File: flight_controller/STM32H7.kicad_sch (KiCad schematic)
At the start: 65 parts, among them SW1 6.0*6.0*6.0, U1 HB-PH9-12727PB2GOB, U2 STM32H743IIT6, X1 XKXEL89CLI-SUAYLC-32.768K, X2 XL2EL89CLI-111YLC-16M

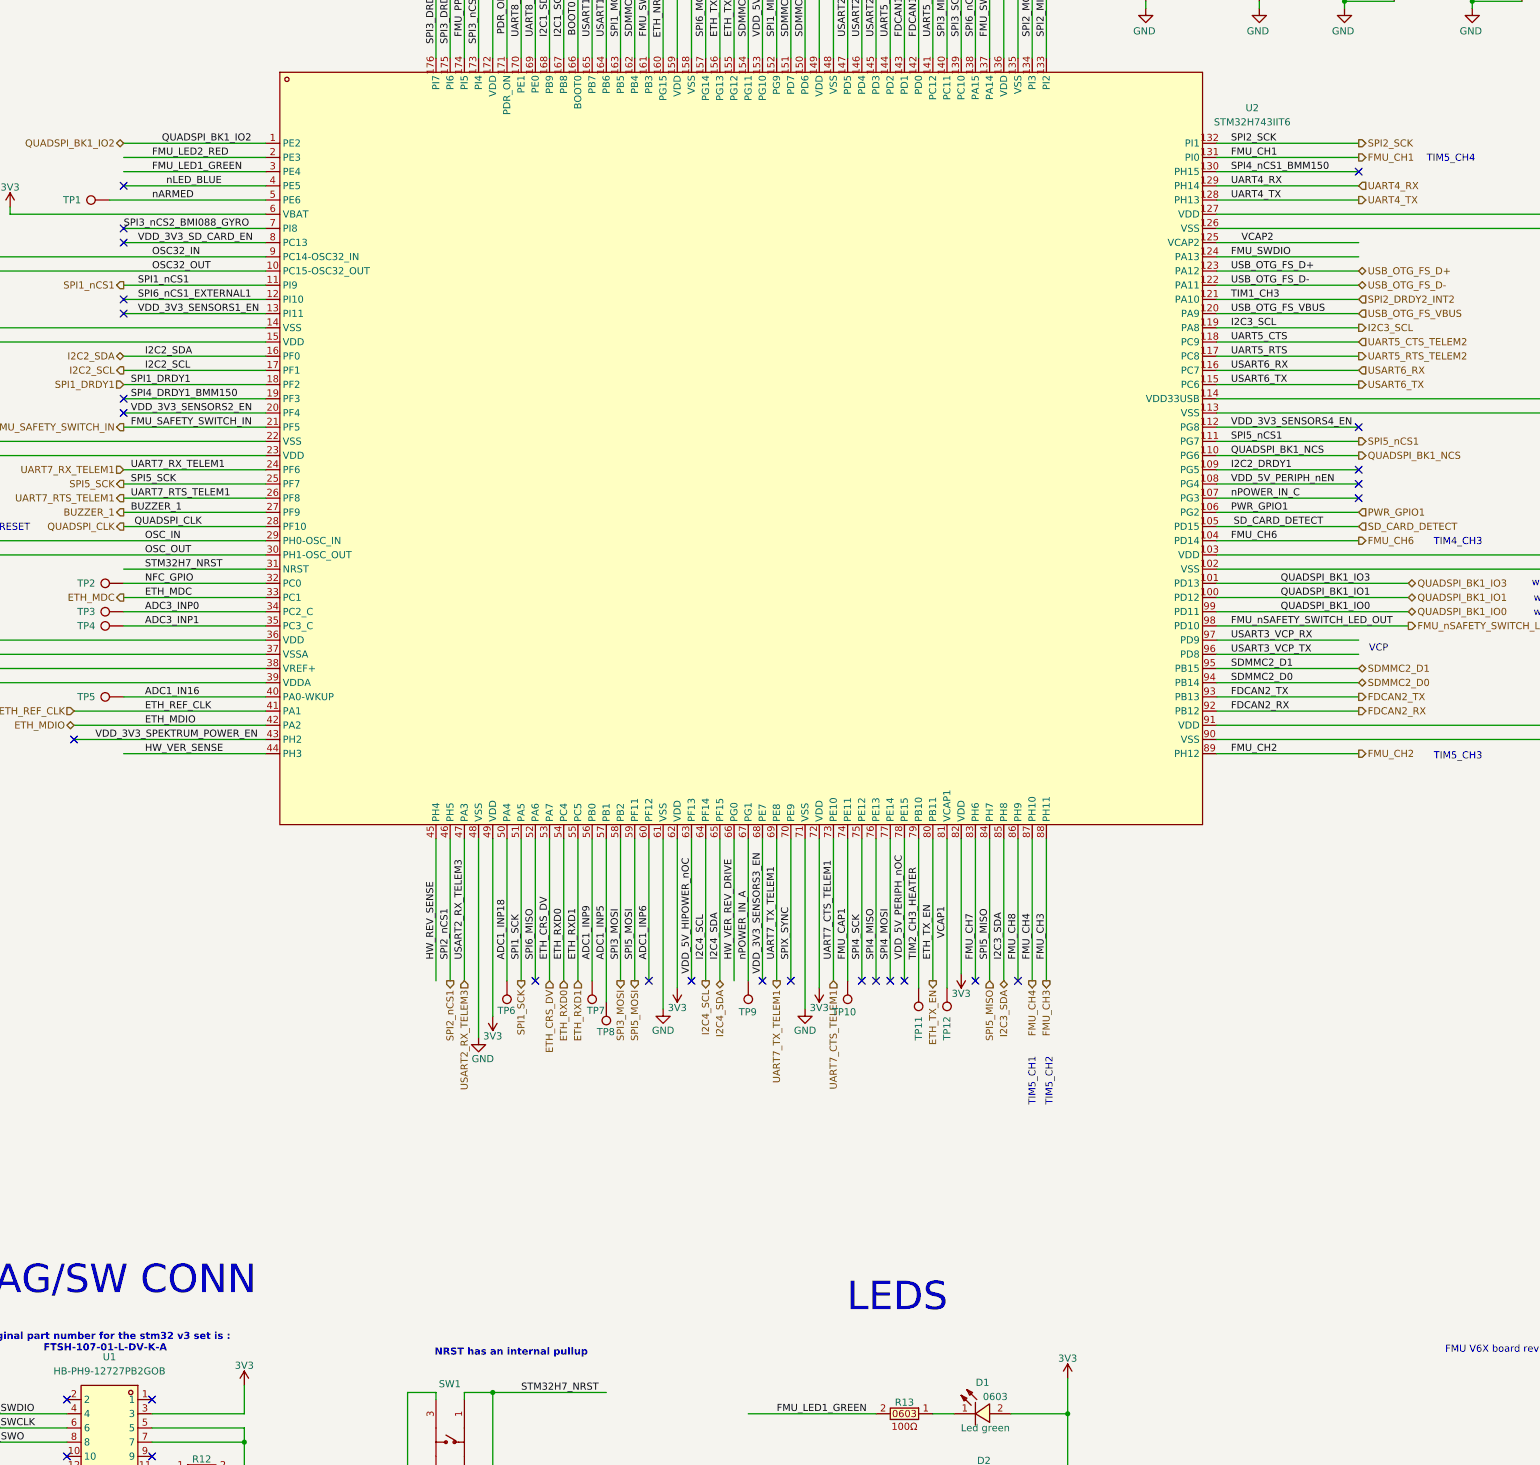
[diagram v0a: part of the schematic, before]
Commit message: Updated power and usb connectors, annotations and netlist check
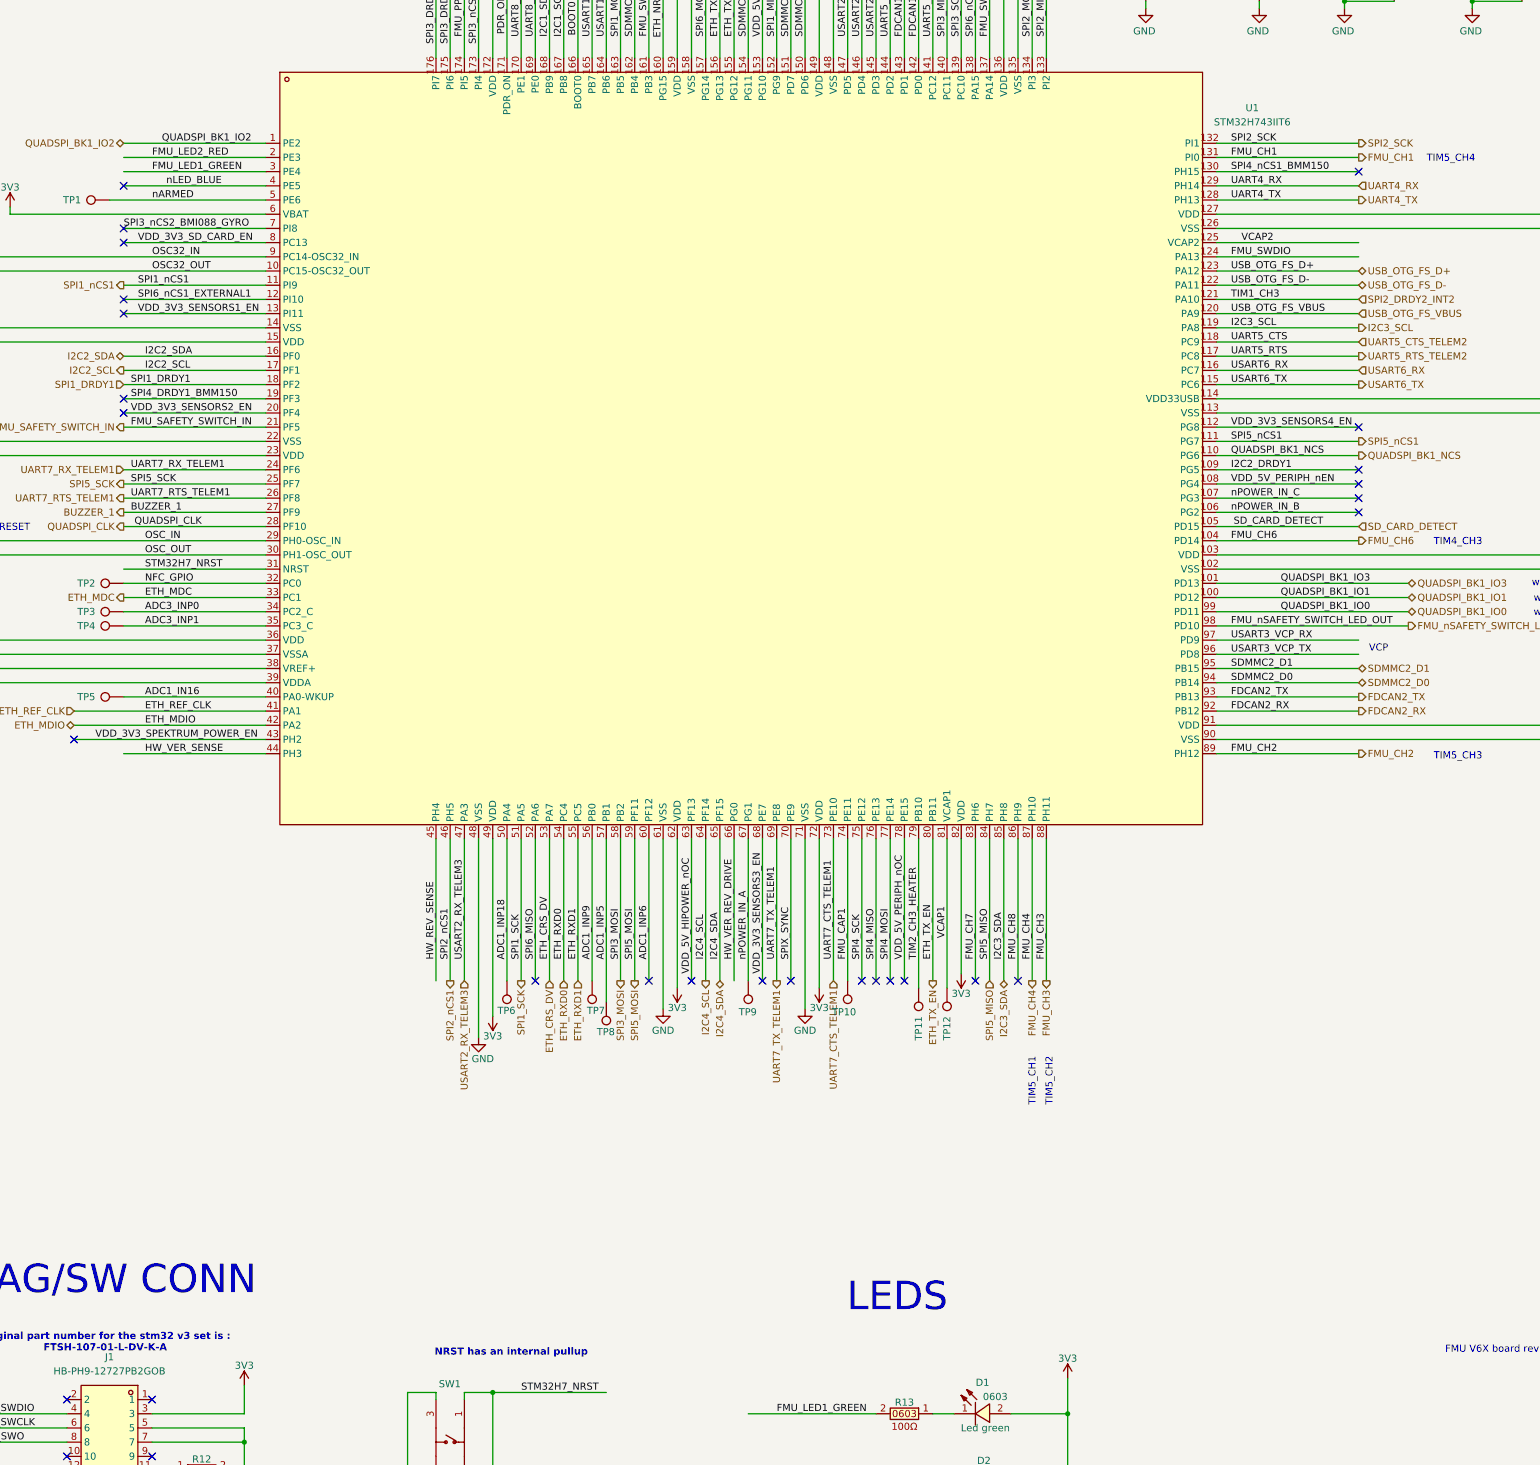
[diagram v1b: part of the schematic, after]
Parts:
- renumbered U1 to J1, U2 to U1
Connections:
- net PWR_GPIO1 renamed nPOWER_IN_B
- no-connect marks 35 -> 36
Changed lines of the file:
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@@
 	)
 	(no_connect
+		(at 511.81 186.69)
+	)
+	(no_connect
 		(at 290.83 166.37)
 	)
@@
 			(width 0)
 			(type default)
+			(color 255 0 0 1)
 		)
 	)
@@
 		)
 	)
-	(label "PWR_GPIO1"
-		(at 488.95 186.69 0)
-		(effects
-			(font
-				(size 1.27 1.27)
-			)
-			(justify left bottom)
-		)
-	)
 	(label "UART5_RX"
 		(at 427.99 101.6 90)
@@
 		)
 	)
+	(label "nPOWER_IN_B"
+		(at 488.95 186.69 0)
+		(effects
+			(font
+				(size 1.27 1.27)
+			)
+			(justify left bottom)
+		)
+	)
 	(label "FMU_SWCLK"
 		(at 445.77 101.6 90)
@@
 		)
 	)
-	(hierarchical_label "PWR_GPIO1"
-		(shape input)
-		(at 511.81 186.69 0)
-		(effects
-			(font
-				(size 1.27 1.27)
-			)
-			(justify left)
-		)
-	)
 	(hierarchical_label "FMU_CH1"
 		(shape output)
@@
 		(on_board yes)
 		(dnp no)
-		(property "Reference" "U1"
+		(property "Reference" "J1"
 			(at 288.29 337.82 0)
 			(effects
@@
 			(project "FP_BOARD"
 				(path "/17737359-1a8e-4237-8899-d9604030bc1d/21c4e215-368e-4a6b-9b68-3566112ef4e7"
-					(reference "U1")
+					(reference "J1")
 					(unit 1)
 				)
@@
 		(dnp no)
 		(fields_autoplaced yes)
-		(property "Reference" "U2"
+		(property "Reference" "U1"
 			(at 492.76 114.3314 0)
 			(effects
@@
 			(project "FP_BOARD"
 				(path "/17737359-1a8e-4237-8899-d9604030bc1d/21c4e215-368e-4a6b-9b68-3566112ef4e7"
-					(reference "U2")
+					(reference "U1")
 					(unit 1)
 				)

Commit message: Revert to state of commit 2458262 moved all to components to top
Reverts commits: d012532, 3d9c600, 58bc0ac
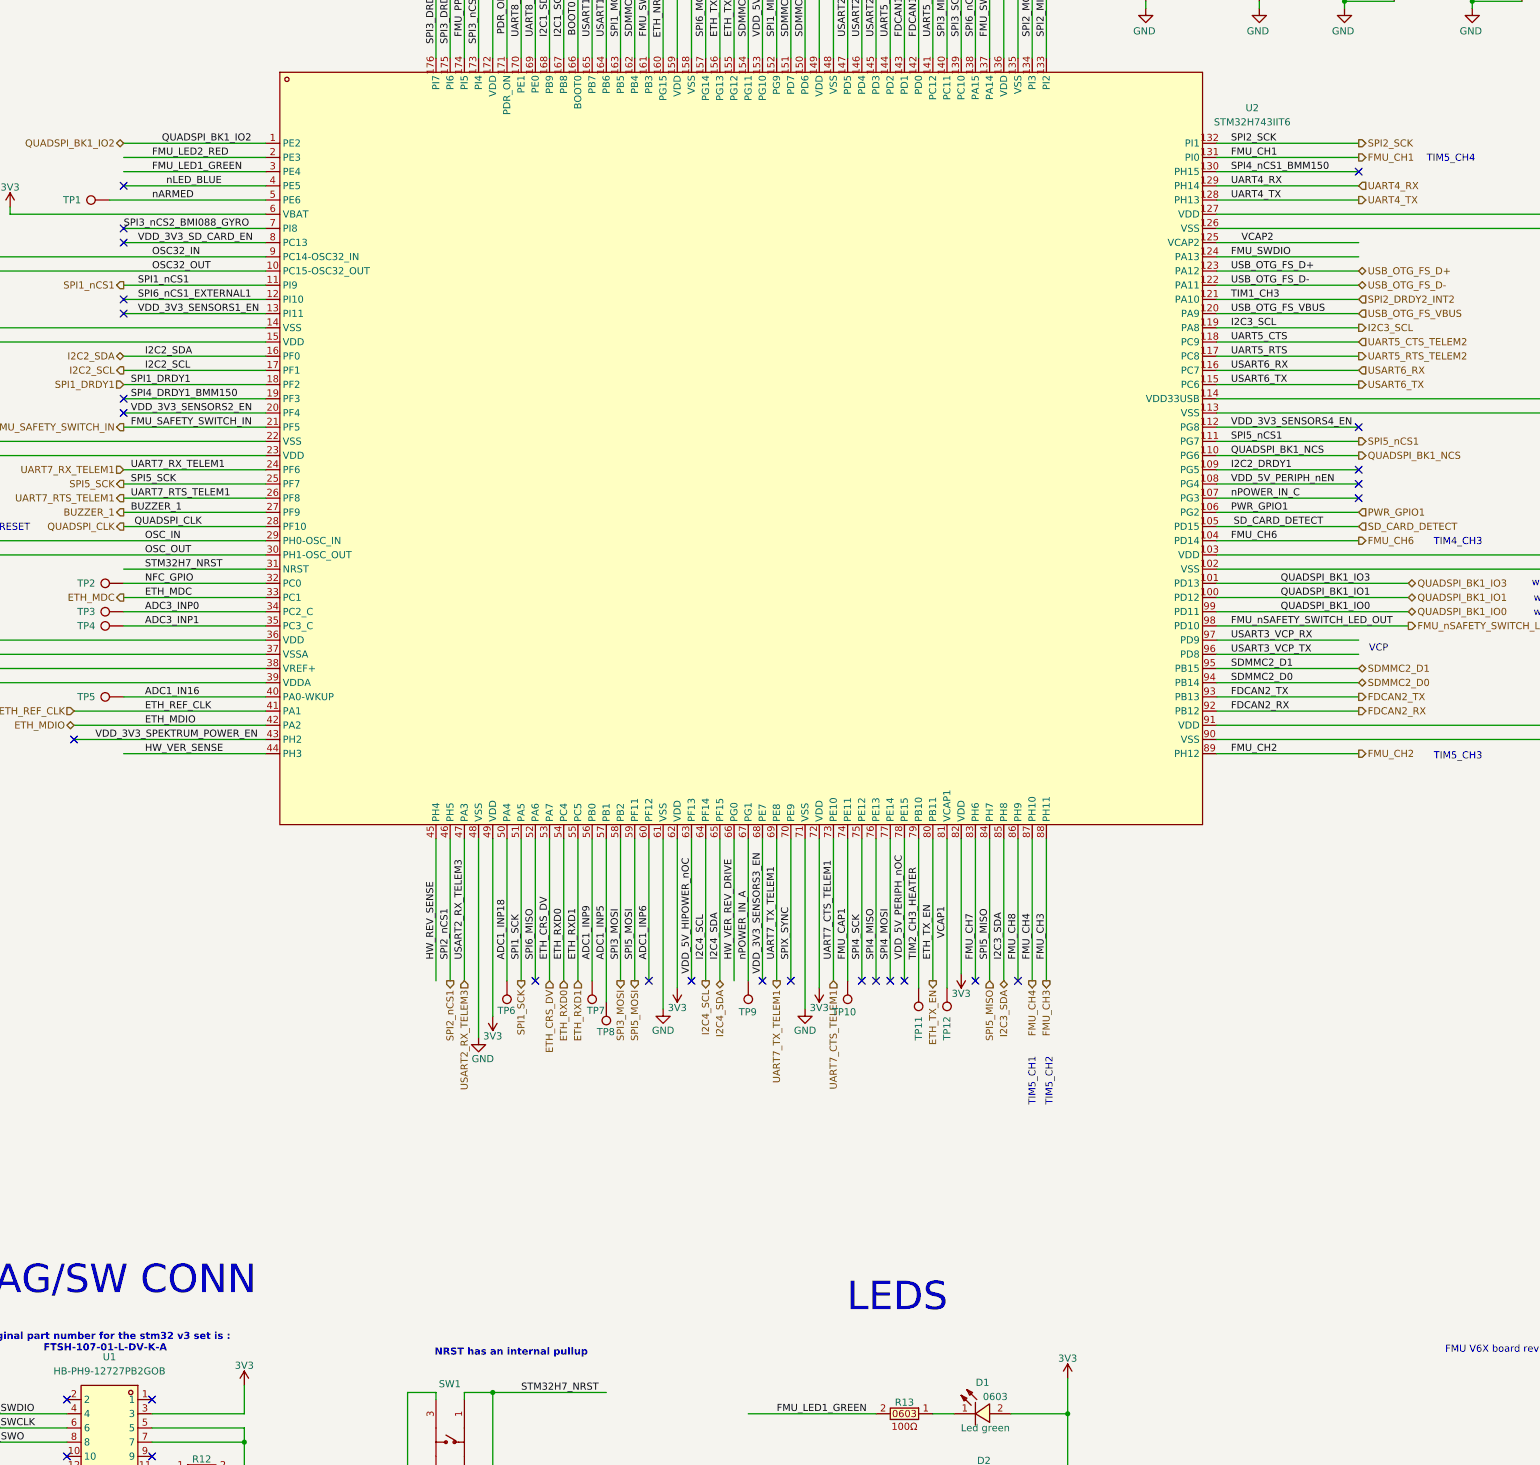
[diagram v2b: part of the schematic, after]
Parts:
- renumbered J1 to U1, U1 to U2
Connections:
- net nPOWER_IN_B renamed PWR_GPIO1
- no-connect marks 36 -> 35
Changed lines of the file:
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@@
 	)
 	(no_connect
-		(at 511.81 186.69)
-	)
-	(no_connect
 		(at 290.83 166.37)
 	)
@@
 			(width 0)
 			(type default)
-			(color 255 0 0 1)
 		)
 	)
@@
 		)
 	)
+	(label "PWR_GPIO1"
+		(at 488.95 186.69 0)
+		(effects
+			(font
+				(size 1.27 1.27)
+			)
+			(justify left bottom)
+		)
+	)
 	(label "UART5_RX"
 		(at 427.99 101.6 90)
@@
 		)
 	)
-	(label "nPOWER_IN_B"
-		(at 488.95 186.69 0)
-		(effects
-			(font
-				(size 1.27 1.27)
-			)
-			(justify left bottom)
-		)
-	)
 	(label "FMU_SWCLK"
 		(at 445.77 101.6 90)
@@
 		)
 	)
+	(hierarchical_label "PWR_GPIO1"
+		(shape input)
+		(at 511.81 186.69 0)
+		(effects
+			(font
+				(size 1.27 1.27)
+			)
+			(justify left)
+		)
+	)
 	(hierarchical_label "FMU_CH1"
 		(shape output)
@@
 		(on_board yes)
 		(dnp no)
-		(property "Reference" "J1"
+		(property "Reference" "U1"
 			(at 288.29 337.82 0)
 			(effects
@@
 			(project "FP_BOARD"
 				(path "/17737359-1a8e-4237-8899-d9604030bc1d/21c4e215-368e-4a6b-9b68-3566112ef4e7"
-					(reference "J1")
+					(reference "U1")
 					(unit 1)
 				)
@@
 		(dnp no)
 		(fields_autoplaced yes)
-		(property "Reference" "U1"
+		(property "Reference" "U2"
 			(at 492.76 114.3314 0)
 			(effects
@@
 			(project "FP_BOARD"
 				(path "/17737359-1a8e-4237-8899-d9604030bc1d/21c4e215-368e-4a6b-9b68-3566112ef4e7"
-					(reference "U1")
+					(reference "U2")
 					(unit 1)
 				)
